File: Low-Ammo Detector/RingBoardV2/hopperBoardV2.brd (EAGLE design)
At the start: 172.2 x 172.3 mm, 17 parts

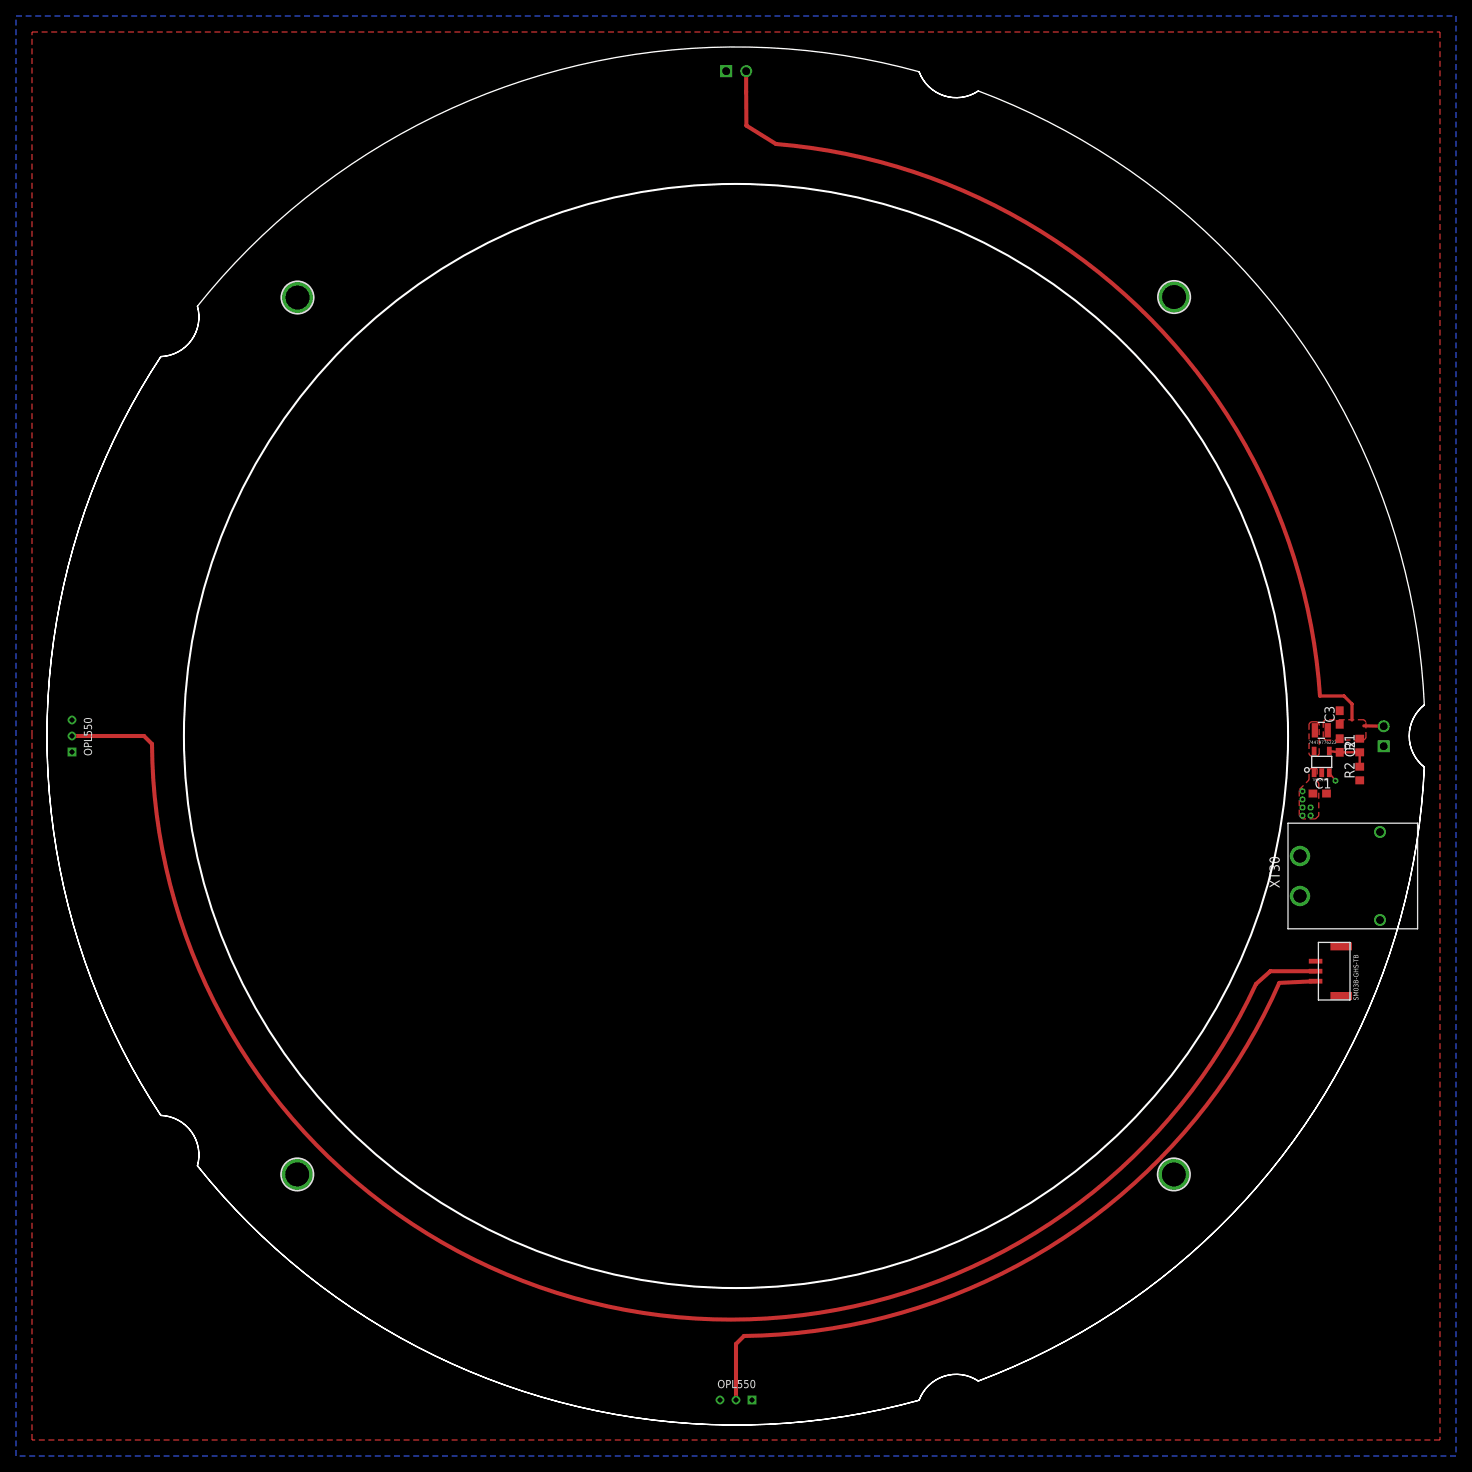
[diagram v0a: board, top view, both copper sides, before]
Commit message: Ammo Board V2
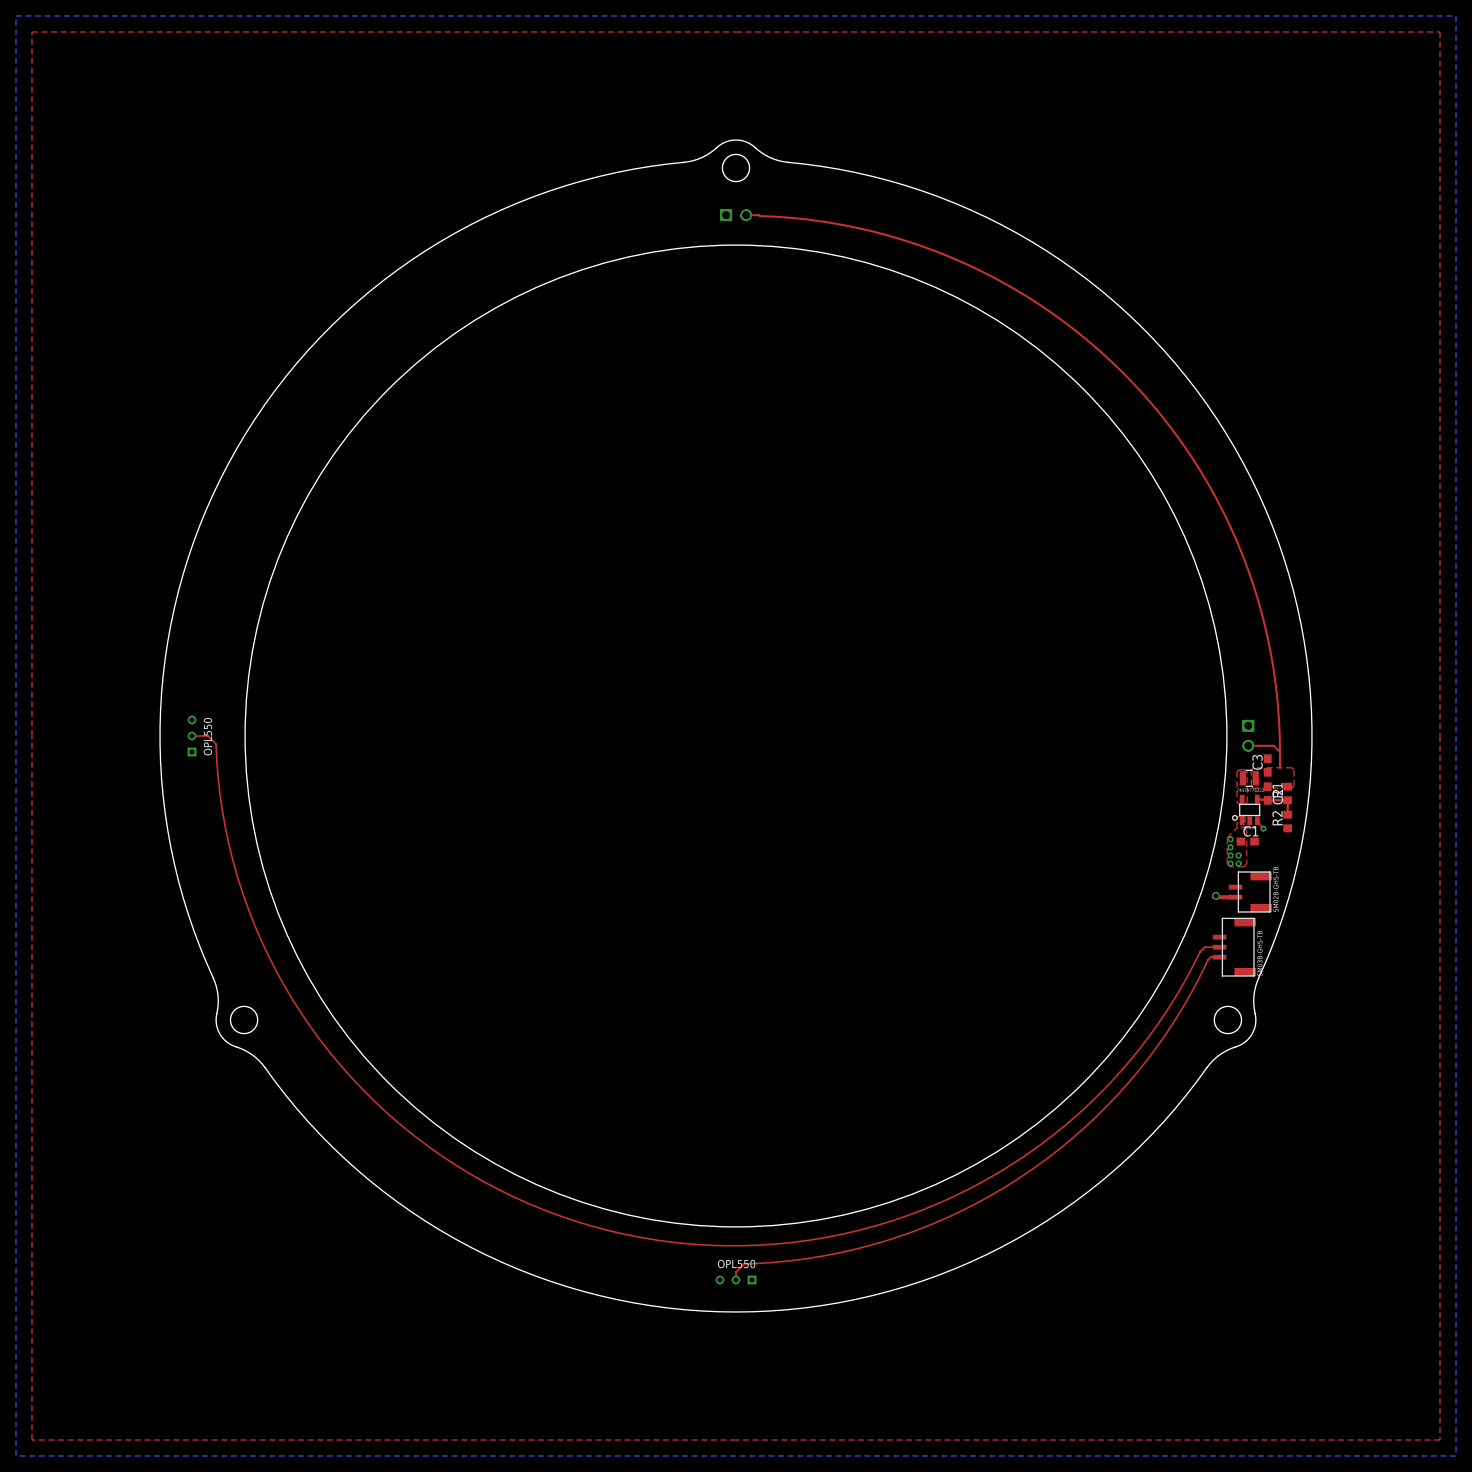
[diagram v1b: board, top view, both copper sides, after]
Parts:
- removed U$10, U$11, U$12, U$7: MOUNTINGHOLE3.0THIN, microbuilder:MOUNTINGHOLE_3.0_PLATEDTHIN
- R1: value 540k -> 330k
- R2: value 360k -> 180k
- U$6: value XT30PW-M -> SM02B-GHS-TB; device _HenrySilva:XT30 -> _HenrySilva:SM02B-GHS-TB
- moved U$2 18.0 mm to (-1.23, 65.1)
- moved U$1 17.1 mm to (64.0, 1.28), turned to 270 degrees
- moved U$3 15.0 mm to (2.00, -68.0)
- moved U$4 15.0 mm to (-68.0, -2.00)
- moved U$8 12.4 mm to (65.0, -30.0)
- moved C1 10.8 mm to (64.0, -13.2)
- moved C2 10.8 mm to (66.5, -7.19)
- moved C3 10.8 mm to (66.5, -3.69)
- moved R1 10.8 mm to (69.0, -7.19)
- moved R2 10.8 mm to (69.0, -10.7)
- moved U$5 10.8 mm to (63.0, -11.2)
- moved U$9 10.8 mm to (63.0, -6.19)
- moved U$6 7.83 mm to (67.0, -22.0), turned to 90 degrees
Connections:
- net 5V: now also U$6.P$3; no longer U$6.P$1
- net GND: now also U$6.P$4; no longer U$6.P$2
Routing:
- net AMMO1: track 159.7 -> 131.8 mm
- net AMMO2: track 93.1 -> 73.3 mm
- net 1.5V: track 116.9 -> 101.4 mm
- net 5V: track 1.26 -> 3.77 mm, vias 7 -> 8
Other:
- board size 172.2 x 172.3 mm -> 144 x 146.5 mm
- board text added: "Purdue Robomaster Ammo Sensor Board V2.0 By Henry Silva 12/7/2019"
- board text removed: "Purdue Robomaster Ammo Sensor Board V1.0 By Henry Silva 11/9/2019"
